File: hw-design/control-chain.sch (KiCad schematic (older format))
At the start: 25 parts, among them J1 RJ45_CHAIN_MAIN, J2 RJ45_CHAIN_EXTENSION, Q1 MMBT3904, Q2 MMBT3906, U4 MAX13450E

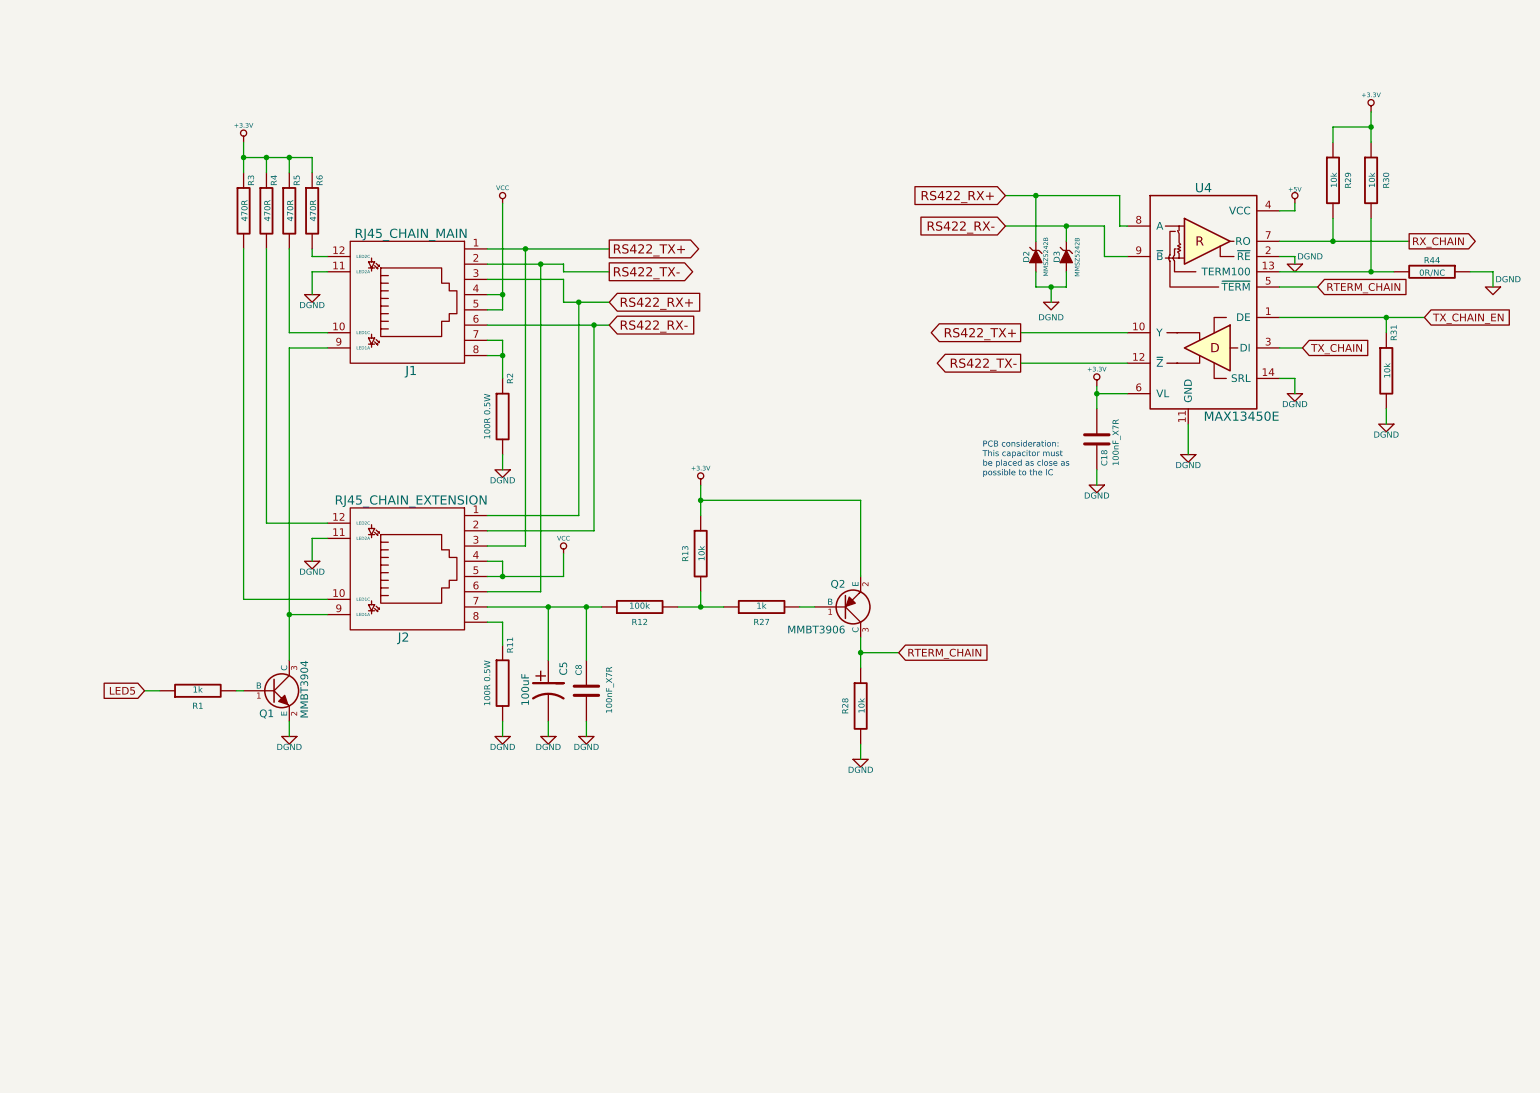
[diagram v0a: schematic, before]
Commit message: using RJ45 leds to indicate cable connection status instead of power status
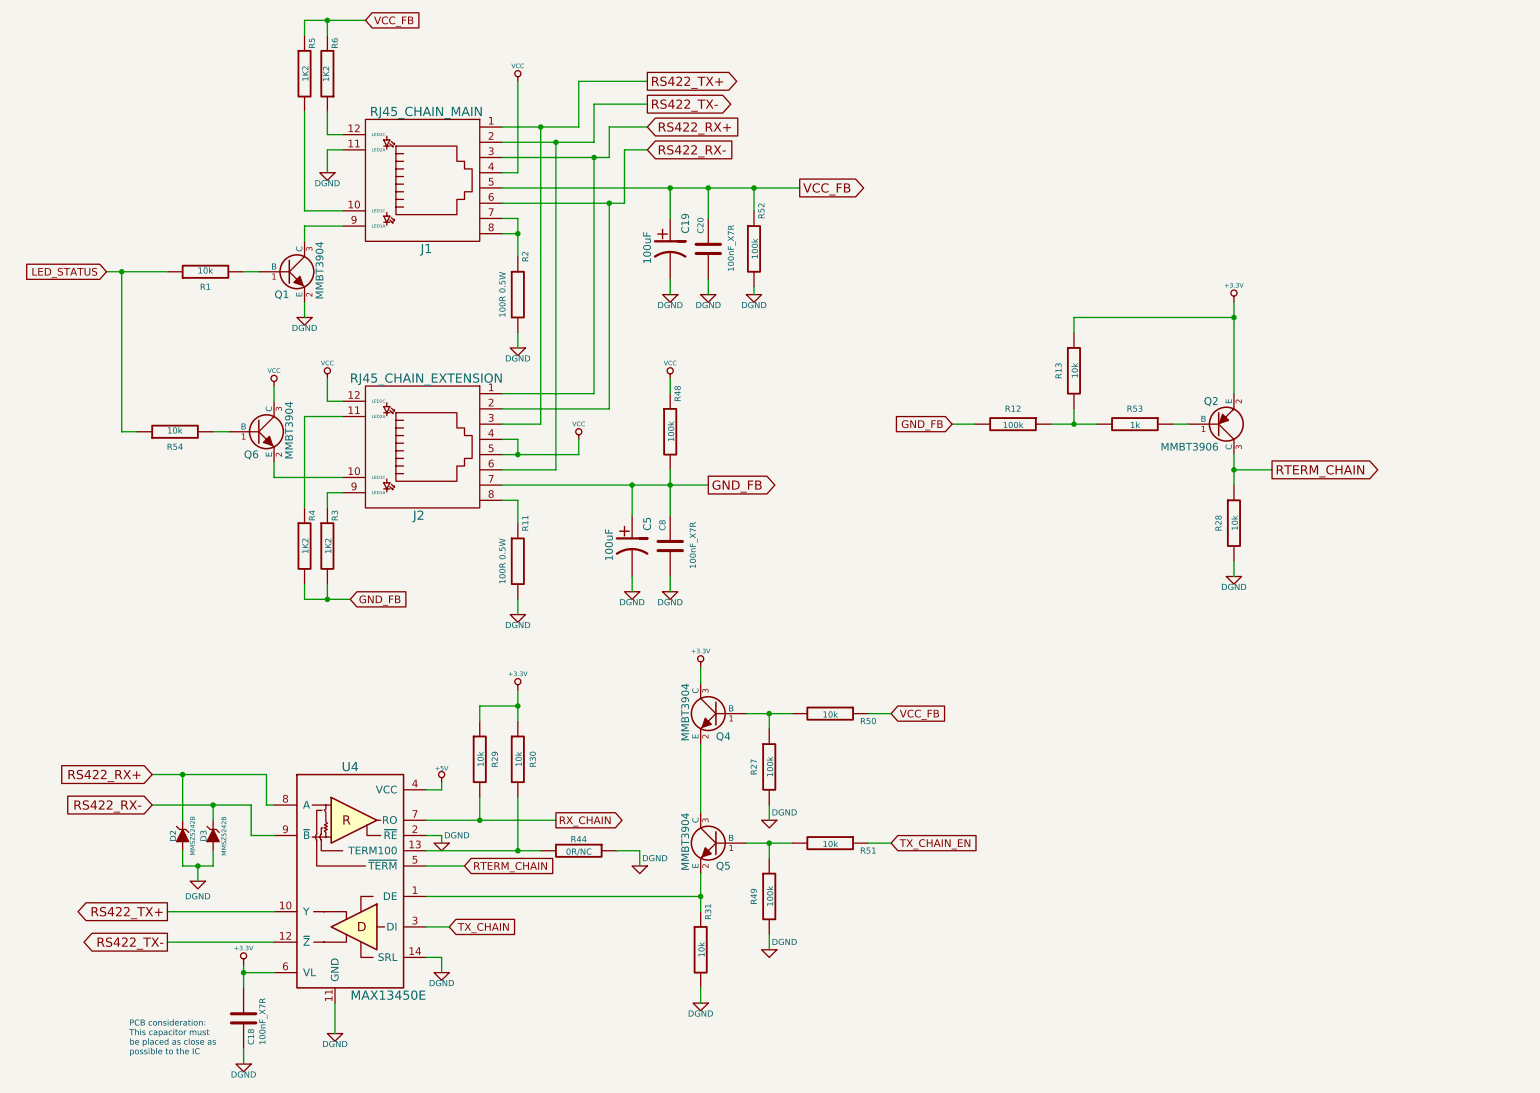
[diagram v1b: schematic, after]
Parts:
- added C19: 100uF, MOD_Footprints_Lib:CAP_RAD_5MM, symbol CP1
- added C20: 100nF_X7R, MOD_Footprints_Lib:SM0603, symbol C
- added Q4, Q5, Q6: MMBT3904, MOD_Footprints_Lib:SOT23, symbol NPN
- added R48, R49, R52: 100k, MOD_Footprints_Lib:SM0603, symbol R
- added R50, R51, R54: 10k, MOD_Footprints_Lib:SM0603, symbol R
- added R53: 1k, MOD_Footprints_Lib:SM0603, symbol R
- R1: value 1k -> 10k
- R12: renamed from R13; value 10k -> 100k
- R13: renamed from R12; value 100k -> 10k
- R27: value 1k -> 100k
- R3, R4, R5, R6: value 470R -> 1K2
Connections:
- net +3.3V: now also R13.1, Q4.3 (C); no longer R12.1, R3.1, R4.1, R5.1, R6.1
- net DGND: now also R27.2, C19.2, C20.2, R49.2, R52.2; no longer J2.11 (LED2A)
- net TX_CHAIN_EN: now also R51.1; no longer R31.1, U4.1 (DE)
- net VCC: now also J2.12 (LED2C), Q6.3 (C), R48.1; no longer J1.5
- net at J1.12 (LED2C): now also R6.1; no longer R6.2
- net at J1.9 (LED1A), Q1.3 (C): no longer J2.9 (LED1A)
- net at J2.10 (LED1C): now also Q6.2 (E); no longer R3.2
- net GND_FB: now reaches R4.2
- net GND_FB: now also C5.1, C8.1, J2.7, R12.2, R3.2, R48.2; no longer J2.12 (LED2C)
- net at Q2.1 (B): now also R53.1; no longer R27.2
- net LED5 renamed LED_STATUS
- net LED_STATUS: now also R54.1
- new net: J2.11 (LED2A), R4.1
- new net: J2.9 (LED1A), R3.1
- new net: Q5.2 (E), R31.1, U4.1 (DE)
- new net: R12.1, R13.2, R53.2
- new net: Q4.1 (B), R27.1, R50.2
- new net: Q4.2 (E), Q5.3 (C)
- new net: Q5.1 (B), R49.1, R51.2
- new net: Q6.1 (B), R54.2
- new net VCC_FB: C19.1, C20.1, J1.5, R5.1, R50.1, R52.1, R6.2
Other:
- moved on the sheet: C18, C5, C8, D2, D3, J1, J2, Q1, Q2, R1, R11, R12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
